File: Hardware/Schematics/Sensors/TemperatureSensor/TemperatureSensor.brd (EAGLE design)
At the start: 15.2 x 19.1 mm, 6 parts, among them Q1 BSS138

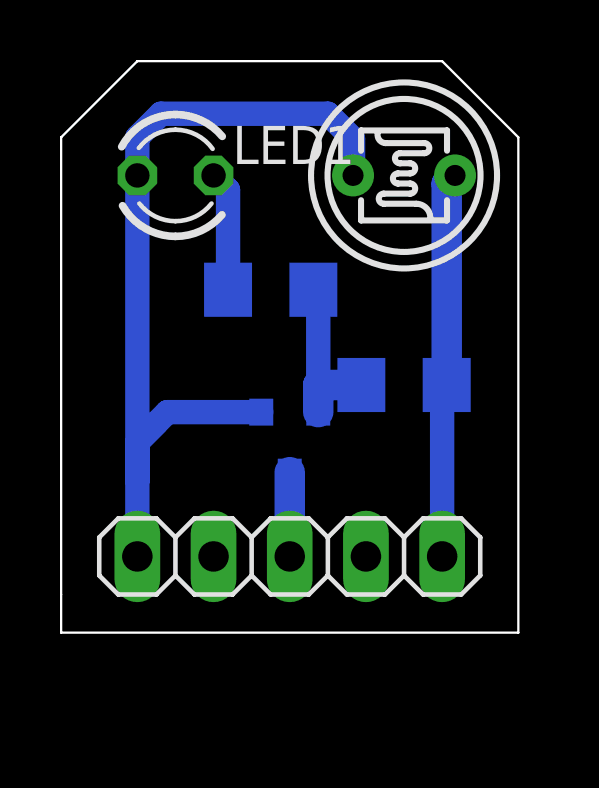
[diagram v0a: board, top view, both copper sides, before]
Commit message: commit
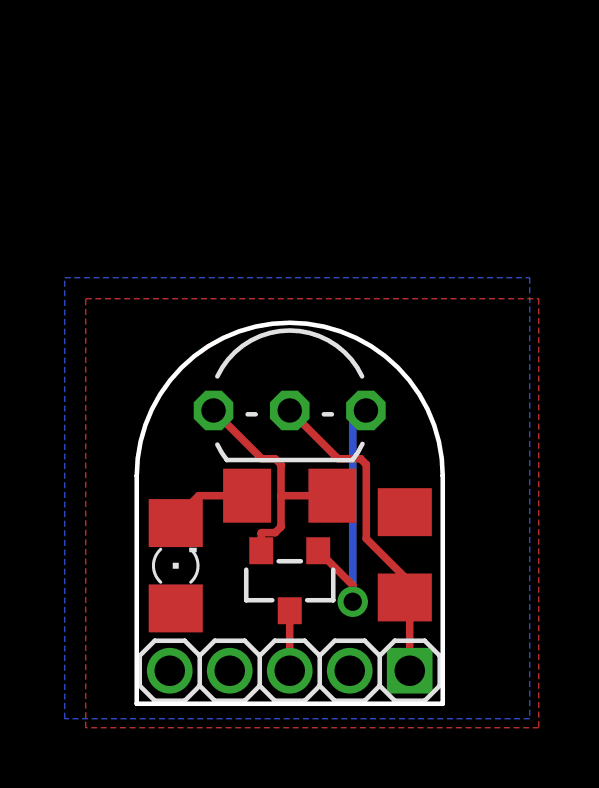
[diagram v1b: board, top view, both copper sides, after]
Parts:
- removed LED1: 3mm 2ma, led:LED3MM
- removed PH1: A10, photo-elements:T0-46-A10XX
- added IC1: DS18B20, 1wire:TO92-
- added LED2: (no value), led:1206
- JP1: device pinhead:1X05 -> pinhead:1_05X2MM
- R1: value 330 -> 1k
- R2: value 1k -> 330
- moved R2 6.89 mm to (0.00, 5.83), flipped to the top, turned to 180 degrees
- moved R1 5.66 mm to (3.83, 3.87), flipped to the top, turned to 270 degrees
- moved Q1 4.62 mm to (0.00, 3.00), flipped to the top
- moved JP1 3.81 mm to (0.00, 0.00)
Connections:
- removed net N$1: JP1.5, LED1.A, PH1.2, Q1.1
- removed net N$13: JP1.1, PH1.1, R1.1
- removed net N$14: Q1.2, R1.2, R2.1
- new net 3V3: IC1.3, JP1.5, LED2.A, Q1.1, R1.1
- new net N$4: IC1.1, Q1.2, R2.1
- new net N$5: IC1.2, JP1.1, R1.2
- net N$2: now also LED2.C; no longer LED1.K
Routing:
- net N$1: track 29.8 -> 0.00 mm
- net N$13: track 12.9 -> 0.00 mm
- net N$5: track 0.00 -> 10.8 mm
- net 3V3: track 0.00 -> 8.73 mm, vias 0 -> 1
- net N$4: track 0.00 -> 8.13 mm
- net N$14: track 5.59 -> 0.00 mm
- net N$2: track 4.01 -> 2.84 mm
- net N$3: track 2.81 -> 2.00 mm
- added copper zone on layer 1, net 3V3
- added copper zone on layer 16, net GND
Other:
- board size 15.2 x 19.1 mm -> 10.2 x 12.7 mm
- board text added: "JLCPCB"
- board text added: "Sponsored"
- board text added: "by"
